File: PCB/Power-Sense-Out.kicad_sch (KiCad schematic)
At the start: 16 parts, among them U9 INA228AIDGSR

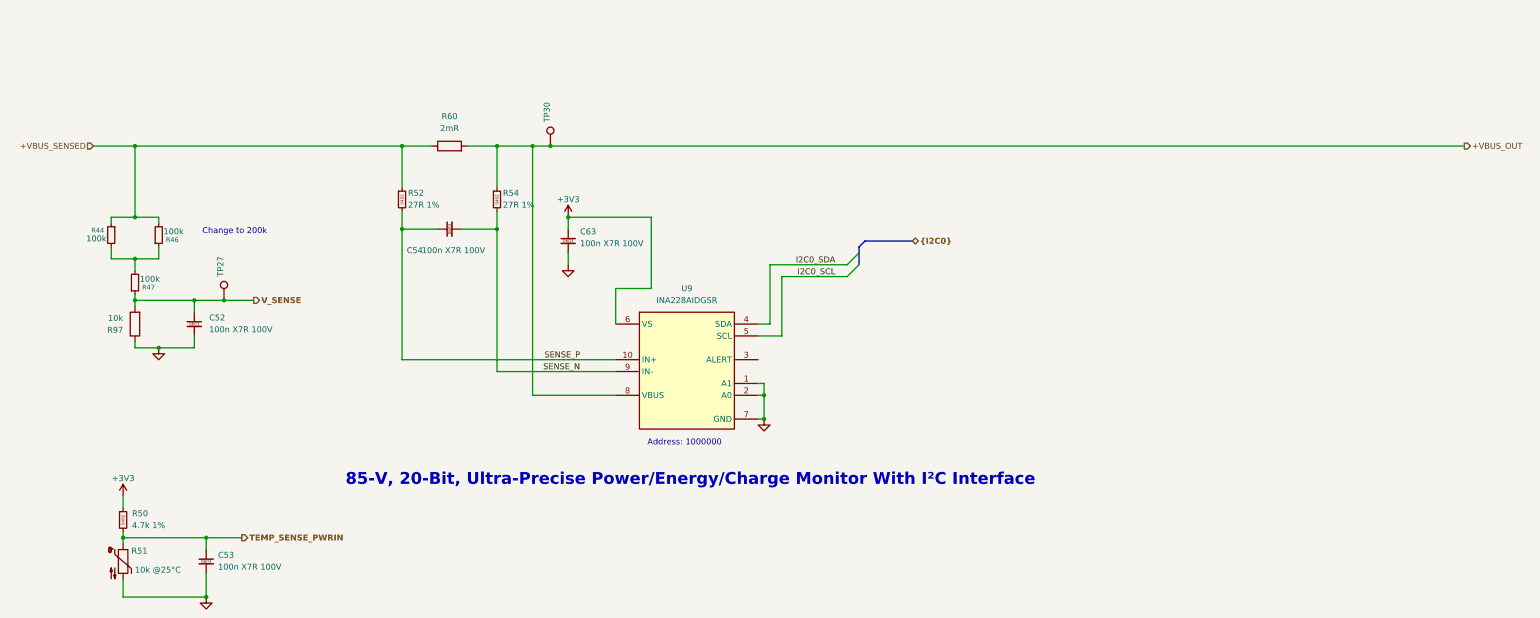
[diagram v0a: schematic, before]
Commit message: Housing Rev3 added
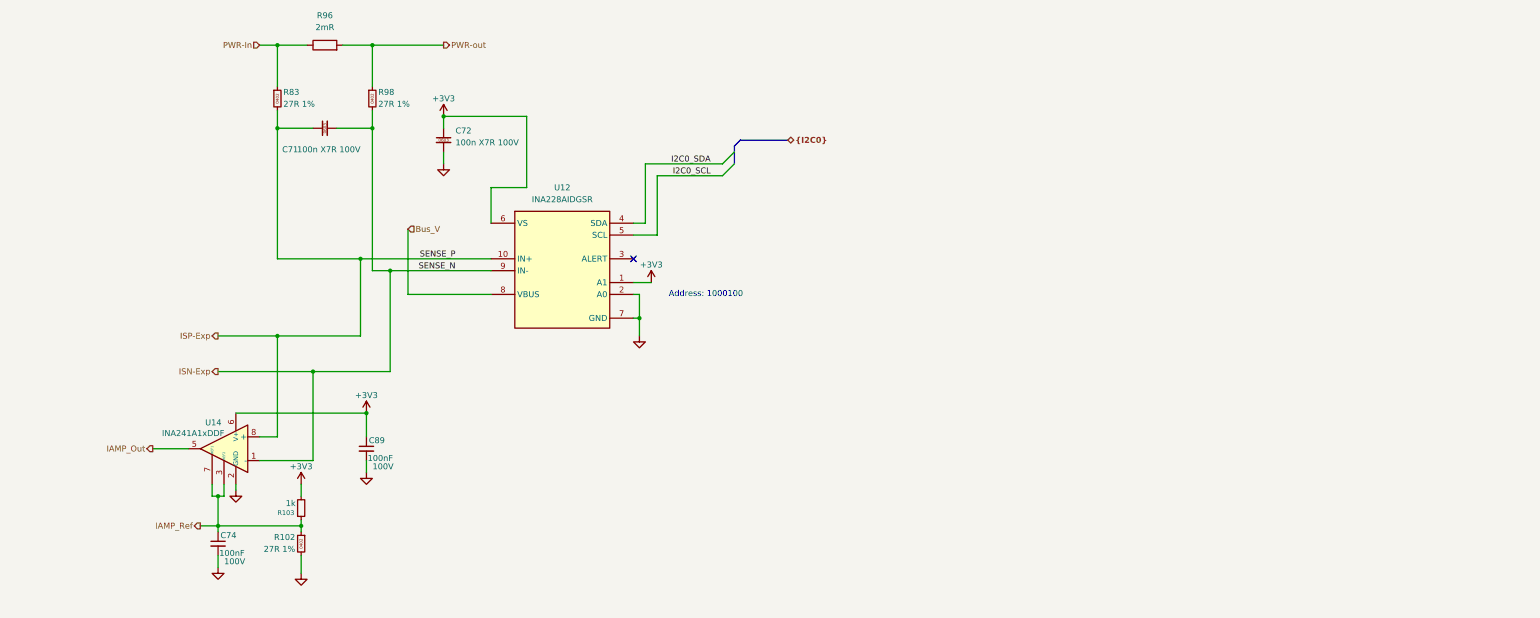
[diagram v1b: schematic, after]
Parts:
- removed C52, C53, C54, C63: 100n X7R 100V, Capacitor_SMD:C_0603_1608Metric, symbol 0_passives:C_0603
- removed R44, R46, R47: 100k, Resistor_SMD:R_0402_1005Metric, symbol Device:R_Small
- removed R50: 4.7k 1%, Resistor_SMD:R_0402_1005Metric, symbol 0_passives:R_0402
- removed R51: 10k @25°C, Resistor_SMD:R_0402_1005Metric, symbol Device:Thermistor_NTC
- removed R52, R54: 27R 1%, Resistor_SMD:R_0402_1005Metric, symbol 0_passives:R_0402
- removed R60: 2mR, Resistor_SMD:R_2512_6332Metric, symbol Device:R
- removed R97: 10k, Resistor_SMD:R_0402_1005Metric, symbol Device:R
- removed TP27, TP30: tp_round_70, TestPoint:TestPoint_Pad_D1.0mm, symbol Connector:TestPoint
- removed U9: INA228AIDGSR, Altium_port:vssop10_50p_300x300x110_mfg, symbol 0_PD240W:INA228AIDGSR
- added C71, C72: 100n X7R 100V, Capacitor_SMD:C_0603_1608Metric, symbol 0_passives:C_0603
- added C74, C89: 100nF, Capacitor_SMD:C_0402_1005Metric, symbol Device:C_Small
- added R102, R83, R98: 27R 1%, Resistor_SMD:R_0402_1005Metric, symbol 0_passives:R_0402
- added R103: 1k, Resistor_SMD:R_0402_1005Metric, symbol Device:R_Small
- added R96: 2mR, Resistor_SMD:R_2512_6332Metric, symbol Device:R
- added U12: INA228AIDGSR, Altium_port:vssop10_50p_300x300x110_mfg, symbol 0_PD240W:INA228AIDGSR
- added U14: INA241A1xDDF, Package_TO_SOT_SMD:SOT-23-8, symbol Amplifier_Current:INA241A1xDDF
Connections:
- net +3V3: now also C72.1, C89.1, R103.2, U12.1 (A1), U12.6 (VS), U14.6 (V+)
- net GND: now also C72.2, C74.2, C89.2, R102.2, U12.2 (A0), U12.7 (GND), U14.2 (GND), U14.4 (GND)
- net I2C0_SCL: now also U12.5 (SCL)
- net I2C0_SDA: now also U12.4 (SDA)
- new net Bus_V: U12.8 (VBUS)
- new net IAMP_Out: U14.5
- new net IAMP_Ref: C74.1, R102.1, R103.1, U14.3 (REF2), U14.7 (REF1)
- new net ISN-Exp: C71.2, R98.2, U12.9 (IN-), U14.1 (-)
- new net ISP-Exp: C71.1, R83.2, U12.10 (IN+), U14.8 (+)
- new net PWR-In: R83.1, R96.1
- new net PWR-out: R96.2, R98.1
- no-connect marks 0 -> 1
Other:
- note added: "Address: 1000100"
- note removed: "85-V, 20-Bit, Ultra-Precise Power/Energy/Charge Monitor With I²C Interface"
- note removed: "Address: 1000000"
- note removed: "Change to 200k"
- title: Nitride-Nano -> (none)
